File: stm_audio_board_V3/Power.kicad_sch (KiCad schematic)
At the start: 66 parts, among them J5 Barrel_Jack_MountingPin, U1 IS42S16100H-7TL, U13 LM7809_TO220, U16 LM7909_TO220, U2 OP275, U4 OP275, U5 MIC2920A-3.3WS-TR, U9 MIC2920A-3.3WS-TR

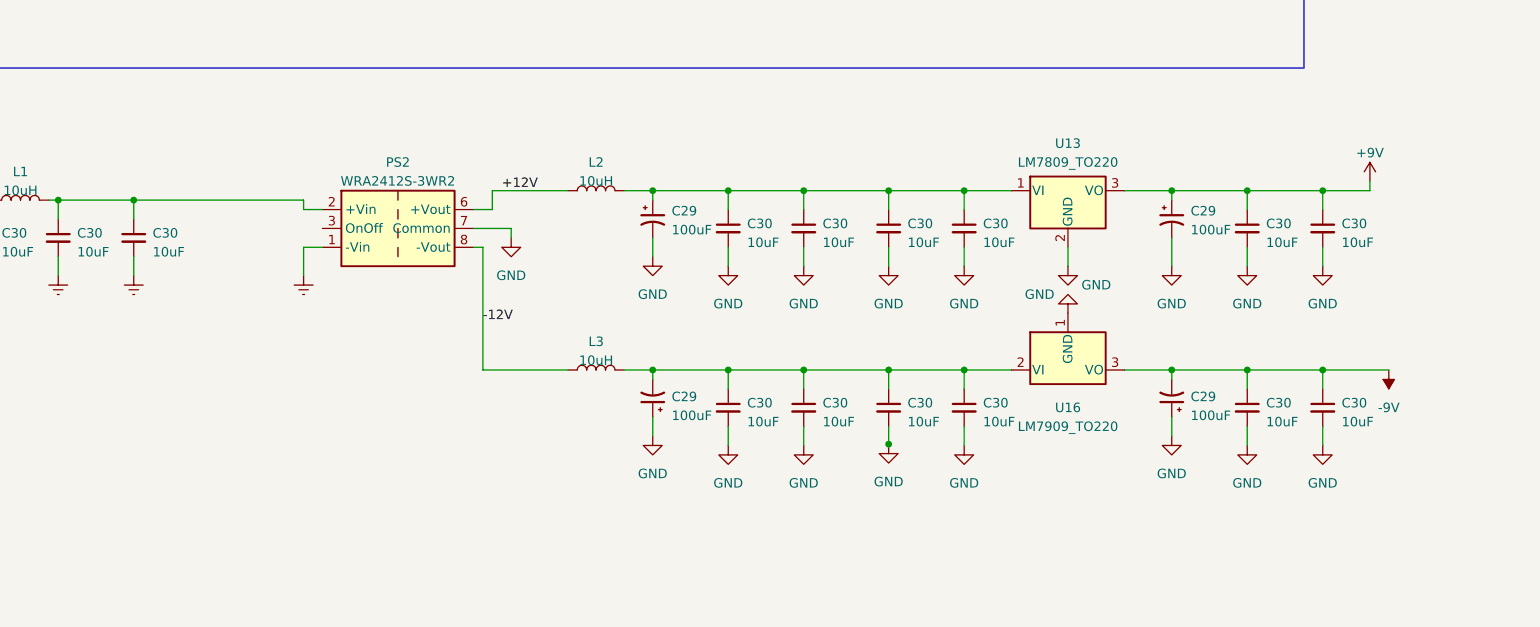
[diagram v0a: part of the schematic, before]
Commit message: safety commit
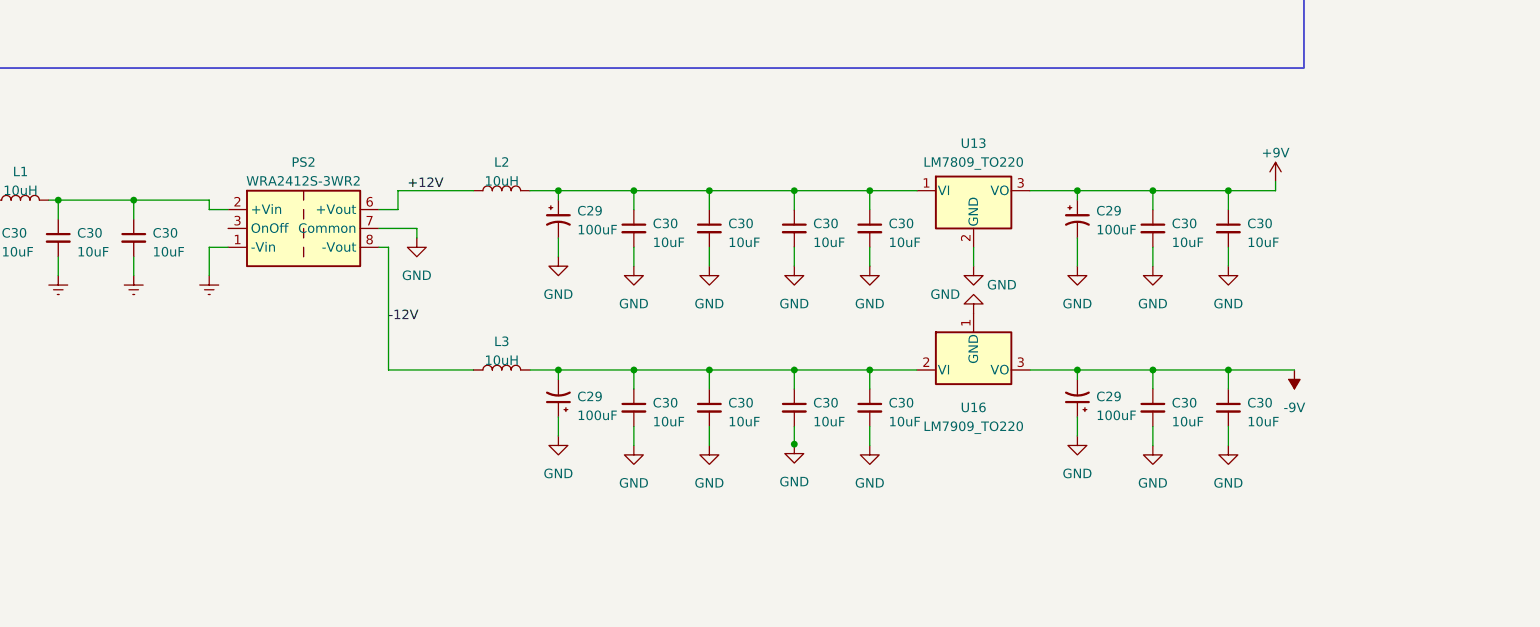
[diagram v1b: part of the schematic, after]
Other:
- moved on the sheet: C29, C30, L2, L3, PS2, U13, U16
